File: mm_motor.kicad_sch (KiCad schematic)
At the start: 2 parts, among them M1 N20_encoder, M3 N20_encoder

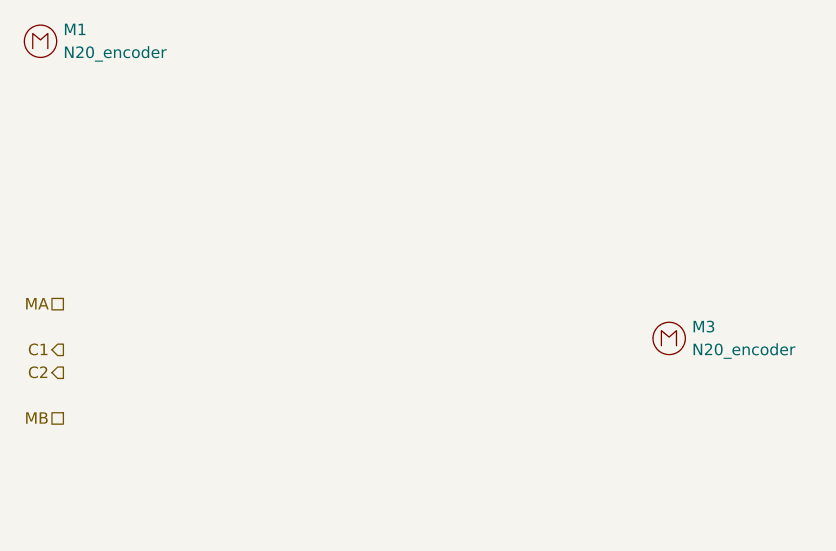
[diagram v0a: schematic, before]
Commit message: tp3
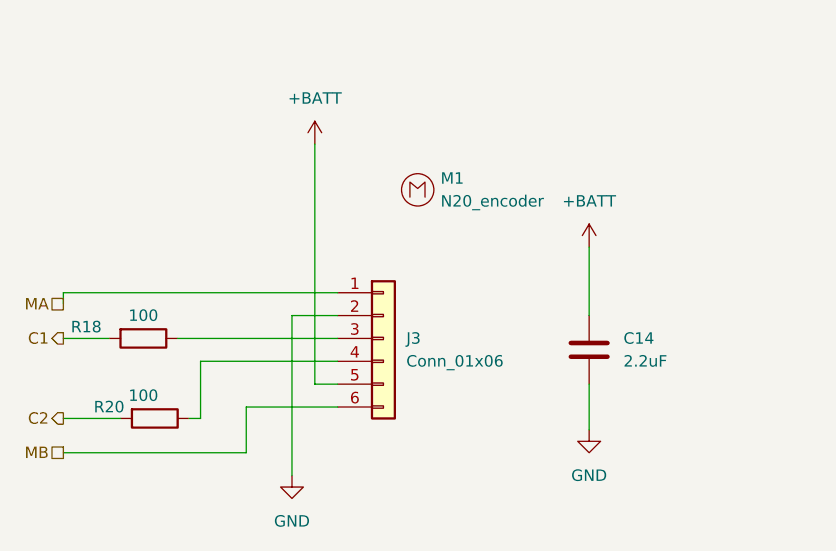
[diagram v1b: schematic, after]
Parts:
- removed M3: N20_encoder, minimouse:N20_with_encoder, symbol minimouse:N20_w_encoder
- added C14: 2.2uF, Capacitor_SMD:C_0603_1608Metric, symbol Device:C
- added J3: Conn_01x06, Connector_PinHeader_2.54mm:PinHeader_1x06_P2.54mm_Vertical, symbol Connector_Generic:Conn_01x06
- added R18, R20: 100, Resistor_SMD:R_0603_1608Metric, symbol Device:R
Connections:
- net C1: now also R18.2
- net C2: now also R20.2
- net MA: now also J3.1 (Pin_1)
- net MB: now also J3.6 (Pin_6)
- new net: J3.4 (Pin_4), R20.1
- new net: J3.3 (Pin_3), R18.1
- new net +BATT: C14.1, J3.5 (Pin_5)
- new net GND: C14.2, J3.2 (Pin_2)
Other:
- moved on the sheet: M1
